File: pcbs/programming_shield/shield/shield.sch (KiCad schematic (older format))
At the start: 20 parts, among them J1 RJ45_LED, J2 RJ45_LED, J3 AVR-ISP-6, P1 Power, P2 Analog, P3 Digital, P4 Digital, U1 MAX489E

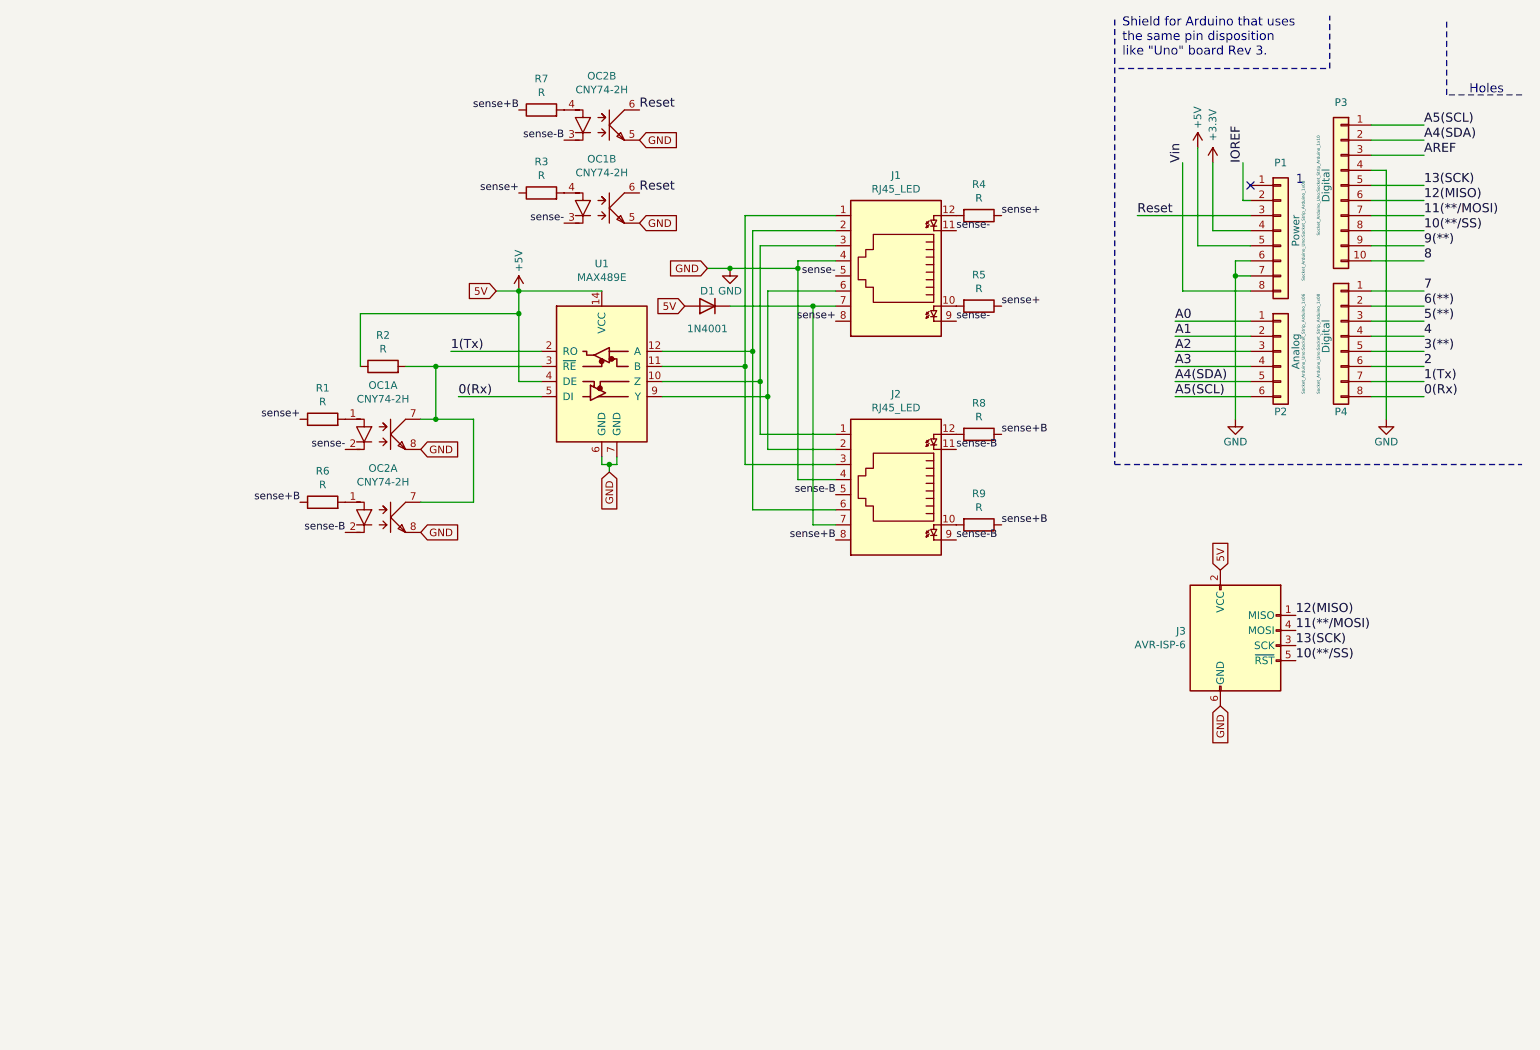
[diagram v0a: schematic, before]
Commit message: revision b of boards
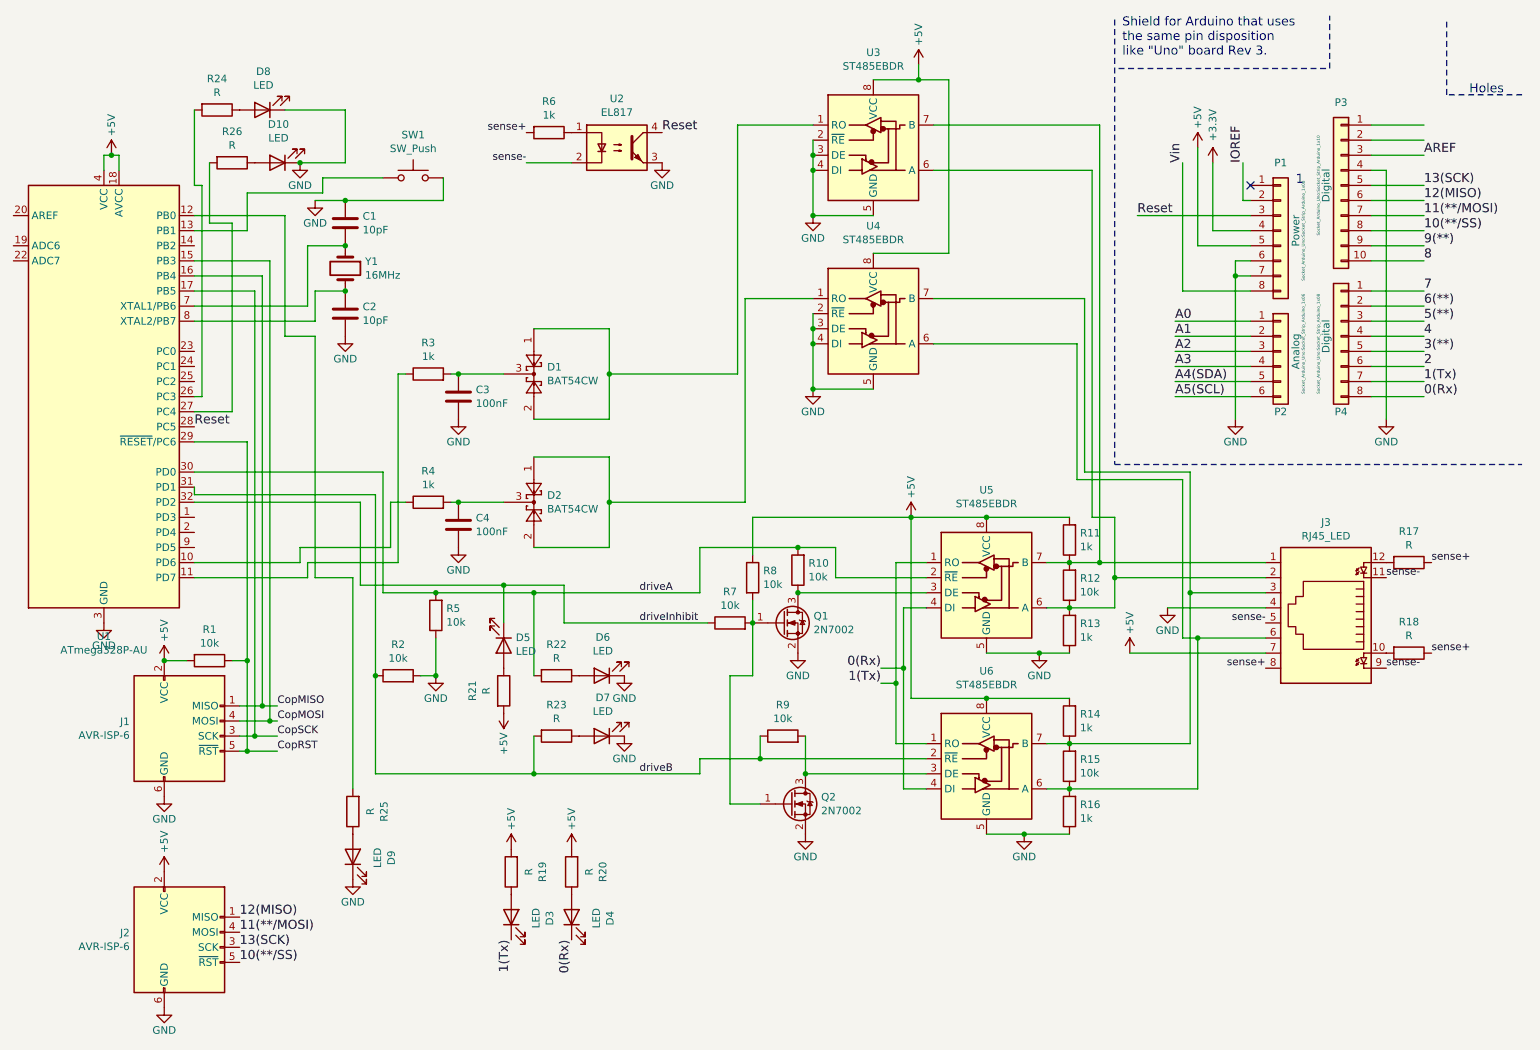
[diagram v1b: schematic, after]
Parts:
- removed D1: 1N4001, Diode_THT:D_DO-41_SOD81_P3.81mm_Vertical_KathodeUp, symbol Diode:1N4001
- removed J2: RJ45_LED, customs:RND_RJ45_LED, symbol Connector:RJ45_LED
- removed OC1, OC2: CNY74-2H, Package_DIP:DIP-8_W7.62mm_LongPads, symbol custom:CNY74-2H
- removed U1: MAX489E, Package_SO:SOIC-14_3.9x8.7mm_P1.27mm, symbol Interface_UART:MAX489E
- added C1, C2: 10pF, Capacitor_SMD:C_0603_1608Metric, symbol Device:C
- added C3, C4: 100nF, Capacitor_THT:C_Disc_D3.0mm_W2.0mm_P2.50mm, symbol Device:C
- added D1, D2: BAT54CW, Package_TO_SOT_SMD:SOT-23, symbol Diode:BAT54CW
- added D10, D3, D4, D5, D6, D7, D8, D9: LED, LED_SMD:LED_0603_1608Metric, symbol Device:LED
- added J1: AVR-ISP-6, Connector_PinSocket_2.54mm:PinSocket_2x03_P2.54mm_Vertical, symbol Connector:AVR-ISP-6
- added Q1, Q2: 2N7002, Package_TO_SOT_SMD:SOT-23, symbol Transistor_FET:2N7002
- added R10, R12, R15, R5: 10k, Resistor_SMD:R_0603_1608Metric, symbol Device:R
- added R11, R13, R14, R16, R4: 1k, Resistor_SMD:R_0603_1608Metric, symbol Device:R
- added R19, R20, R21, R22, R23, R24, R25, R26: R, Resistor_SMD:R_0603_1608Metric, symbol Device:R
- added SW1: SW_Push, Button_Switch_THT:SW_PUSH_6mm, symbol Switch:SW_Push
- added U1: ATmega328P-AU, Package_QFP:TQFP-32_7x7mm_P0.8mm, symbol MCU_Microchip_ATmega:ATmega328P-AU
- added U2: EL817, Package_DIP:DIP-4_W7.62mm, symbol Isolator:EL817
- added U3, U4, U5, U6: ST485EBDR, Package_SO:SOIC-8_3.9x4.9mm_P1.27mm, symbol Interface_UART:ST485EBDR
- added Y1: 16MHz, Crystal:Crystal_HC49-4H_Vertical, symbol Device:Crystal
- R1, R2, R7, R8, R9: value R -> 10k
- R3, R6: value R -> 1k
- renumbered J3 to J2, J1 to J3, R4 to R17, R5 to R18
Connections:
- net +5V: now also J3.7, R1.2, R8.1, J1.2 (VCC), R11.2, R14.2, R19.2, R20.2, R21.2, U1.18 (AVCC), U1.4 (VCC), U1.6 (VCC), U3.8 (VCC), U4.8 (VCC), U5.8 (VCC), U6.8 (VCC); no longer R2.1
- net 0(Rx): now also D4.1 (K), U5.4 (DI), U6.4 (DI)
- net 1(Tx): now also D3.1 (K), U5.1 (RO), U6.1 (RO)
- net A4(SDA): no longer P3.2 (Pin_2)
- net A5(SCL): no longer P3.1 (Pin_1)
- net GND: now also R2.2, C1.1, C2.2, C3.2, C4.2, D10.1 (K), D6.1 (K), D7.1 (K), D8.1 (K), D9.1 (K), J1.6 (GND), Q1.2 (S), Q2.2 (S), R13.1, R16.1, R5.1, SW1.2, U1.21 (GND), U1.3 (GND), U1.5 (GND), U2.3, U3.2 (~RE), U3.3 (DE), U3.4 (DI), U3.5 (GND), U4.2 (~RE), U4.3 (DE), U4.4 (DI), U4.5 (GND), U5.5 (GND), U6.5 (GND)
- net Reset: now also U1.28 (PC5), U2.4
- net sense+: now also R6.2; no longer R1.1, R3.1
- net sense-: now also U2.2
- net at J3.3: now also R14.1, R15.2, U4.7 (B), U6.7 (B)
- net at J3.1: now also R11.1, R12.2, U3.7 (B), U5.7 (B)
- net at J3.2: now also R12.1, R13.2, U3.6 (A), U5.6 (A)
- net at J3.6: now also R15.1, R16.2, U4.6 (A), U6.6 (A)
- net at R3.2: now also C3.1, D1.3
- net at R9.2: now also Q2.3 (D), U6.3 (DE)
- net at R8.2: now also R7.2, Q1.1 (G), Q2.1 (G)
- removed net sense+B: R6.1, R7.1, R8.1, R9.1
- new net: Q1.3 (D), R10.1, U5.3 (DE)
- new net: C1.2, U1.7 (XTAL1/PB6), Y1.1
- new net: C2.1, U1.8 (XTAL2/PB7), Y1.2
- new net: D1.1, D1.2, U3.1 (RO)
- new net: R3.1, U1.11 (PD7)
- new net: C4.1, D2.3, R4.2
- new net: D2.1, D2.2, U4.1 (RO)
- new net: R4.1, U1.10 (PD6)
- new net: R6.1, U2.1
- new net: R25.2, U1.12 (PB0)
- new net: SW1.1, U1.13 (PB1)
- new net: R24.2, U1.26 (PC3)
- new net: R26.2, U1.27 (PC4)
- new net: D3.2 (A), R19.1
- new net: D4.2 (A), R20.1
- new net: D6.2 (A), R22.1
- new net: D7.2 (A), R23.1
- new net: D8.2 (A), R24.1
- new net: D5.2 (A), R21.1
- new net: D9.2 (A), R25.1
- new net: D10.2 (A), R26.1
- new net CopMISO: J1.1 (MISO), U1.16 (PB4)
- new net CopMOSI: J1.4 (MOSI), U1.15 (PB3)
- new net CopRST: J1.5 (~RST), R1.1, U1.29 (~RESET~/PC6)
- new net CopSCK: J1.3 (SCK), U1.17 (PB5)
- new net driveA: R10.2, R22.2, R5.2, U1.30 (PD0), U5.2 (~RE)
- new net driveB: R2.1, R23.2, R9.1, U1.31 (PD1), U6.2 (~RE)
- new net driveInhibit: D5.1 (K), R7.1, U1.32 (PD2)
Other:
- moved on the sheet: J2, J3, R17, R18
